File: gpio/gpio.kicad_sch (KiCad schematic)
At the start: 17 parts, among them J1 Screw Termial, J2 Screw Terminal, J3 Screw Termial, J4 Screw Termial, J5 I2C, J6 RotaryEncoder, U1 VoltageRegulator, U2 ESP32, U3 TJA1050

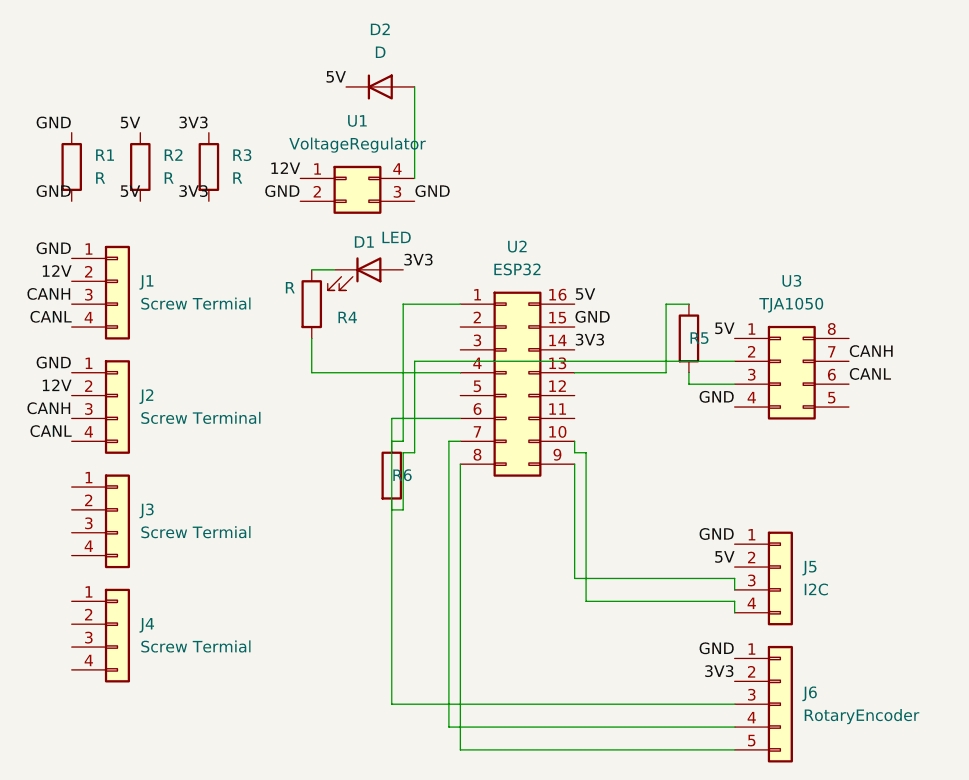
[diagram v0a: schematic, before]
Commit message: gpio
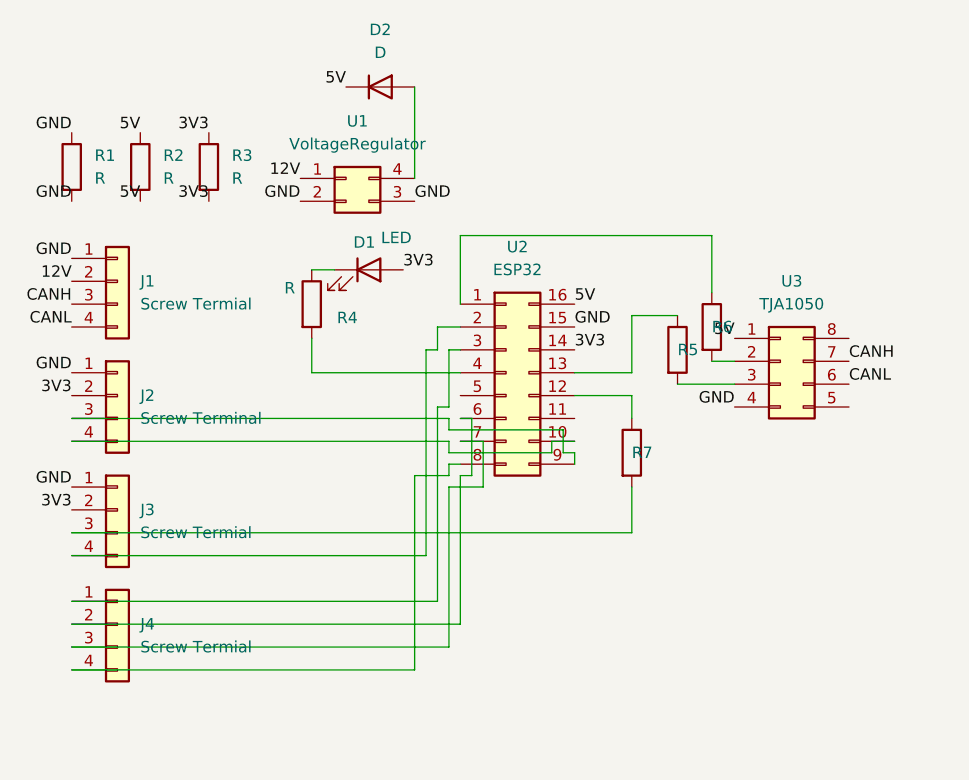
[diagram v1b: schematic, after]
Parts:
- removed J5: I2C, Peabrain:I2C_Connector, symbol Connector_Generic:Conn_01x04
- removed J6: RotaryEncoder, Peabrain:RotaryEncoderConnection, symbol Connector_Generic:Conn_01x05
- added R7: ~, Resistor_THT:R_Axial_DIN0207_L6.3mm_D2.5mm_P10.16mm_Horizontal, symbol Device:R
- R6: value (none) -> ~
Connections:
- net 12V: no longer J2.2 (Pin_2)
- net 3V3: now also J2.2 (Pin_2), J3.2 (Pin_2)
- net CANH: no longer J2.3 (Pin_3)
- net CANL: no longer J2.4 (Pin_4)
- net GND: now also J3.1 (Pin_1)
- net at U2.9 (Pin_9): now also J2.3 (Pin_3)
- net at U2.10 (Pin_10): now also J2.4 (Pin_4)
- net at U2.12 (Pin_12): now also R7.1
- net at U2.2 (Pin_2): now also J3.4 (Pin_4)
- net at U2.3 (Pin_3): now also J4.1 (Pin_1)
- net at U2.6 (Pin_6): now also J4.2 (Pin_2)
- net at U2.7 (Pin_7): now also J4.3 (Pin_3)
- net at U2.8 (Pin_8): now also J4.4 (Pin_4)
- net at J3.3 (Pin_3): now also R7.2
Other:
- moved on the sheet: R5
